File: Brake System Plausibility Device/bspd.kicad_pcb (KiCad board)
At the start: 2 copper layers, 87.9 x 41.3 mm, 29 parts, among them P1 MX150_16, SW1 RESET, U1 MCP604, U2 LM1117-5.0, U3 74LVC2G74, U4 74AUC2G00

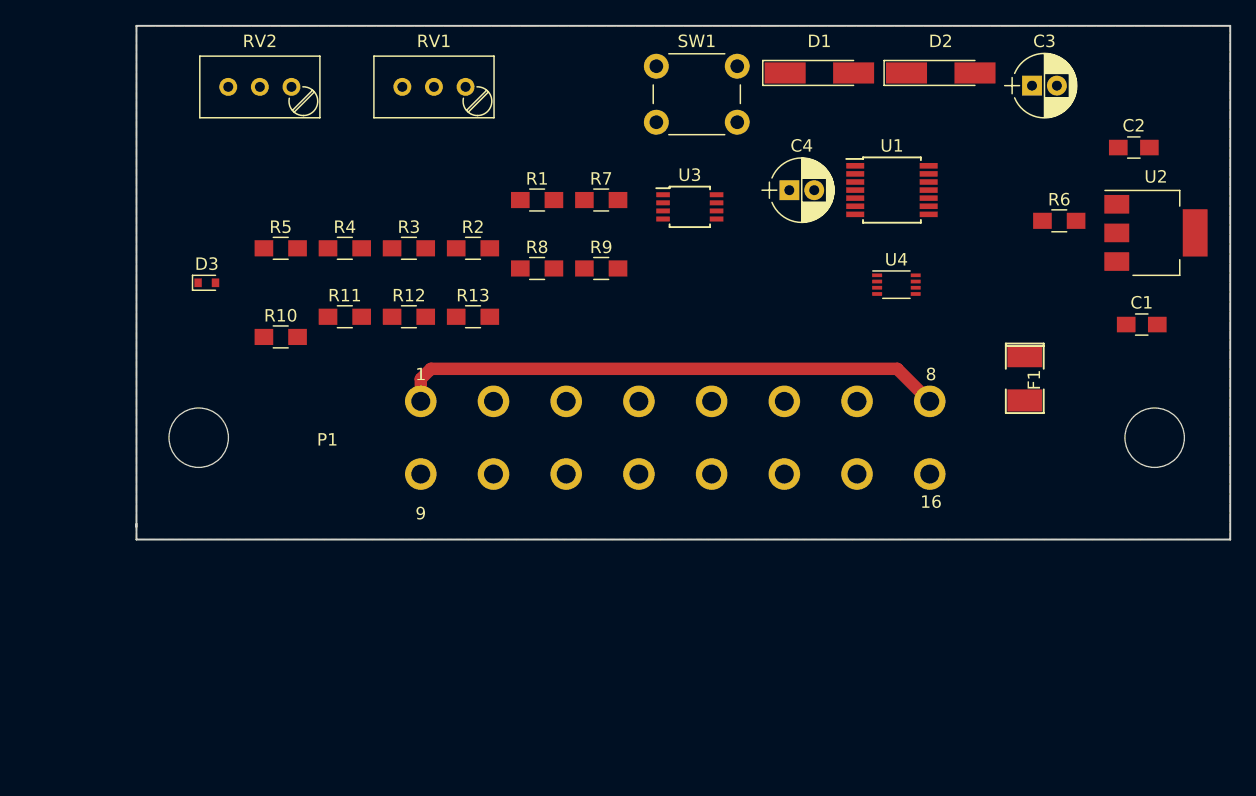
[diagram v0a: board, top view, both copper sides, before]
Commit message: BSPD Layout Done
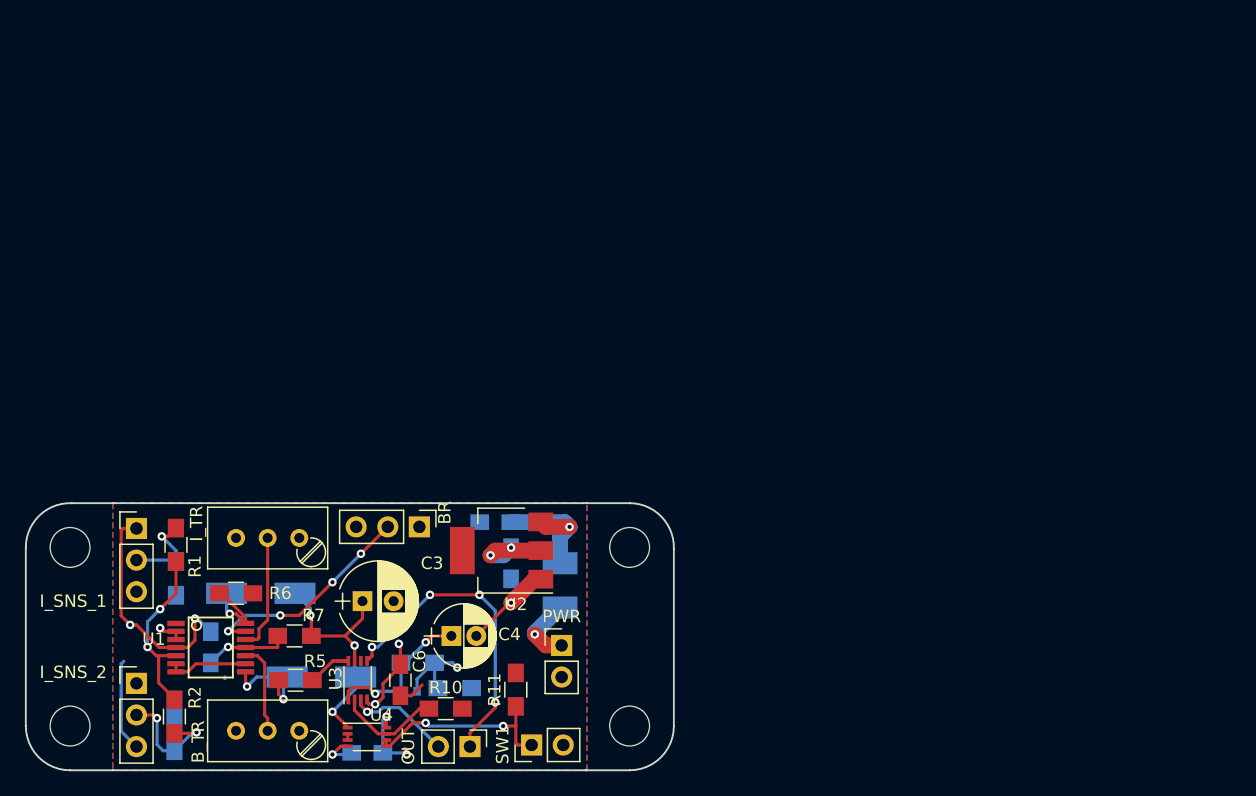
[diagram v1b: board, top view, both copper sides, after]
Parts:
- removed P1: MX150_16, UNCAMotorsports:MX150_16pin
- removed R12, R13: 1k, Resistors_SMD:R_0805_HandSoldering
- removed RV1: 5KW trim - 10k, Potentiometers:Potentiometer_Trimmer_Bourns_3296W
- removed RV2: Braking trim - 10k, Potentiometers:Potentiometer_Trimmer_Bourns_3296W
- added BR: BRAKE_SENSOR, Pin_Headers:Pin_Header_Straight_1x03_Pitch2.54mm, F.Cu at (133.0, 88.8)
- added B_TR: 5KW trim - 10k, Potentiometers:Potentiometer_Trimmer_Bourns_3296W, F.Cu at (123.3, 105.2)
- added C5: 1u, Capacitors_SMD:C_0805_HandSoldering, B.Cu at (116.2, 98.4)
- added C6: 1u, Capacitors_SMD:C_0805_HandSoldering, F.Cu at (131.4, 101.1)
- added C7: 1u, Capacitors_SMD:C_0805_HandSoldering, B.Cu at (128.8, 106.9)
- added I_SNS_1: CURRENT_SENSE_2, Pin_Headers:Pin_Header_Straight_1x03_Pitch2.54mm, F.Cu at (110.2, 88.9)
- added I_SNS_2: CURRENT_SENSE_1, Pin_Headers:Pin_Header_Straight_1x03_Pitch2.54mm, F.Cu at (110.2, 101.3)
- added I_TR: Braking trim - 10k, Potentiometers:Potentiometer_Trimmer_Bourns_3296W, F.Cu at (123.3, 89.7)
- added OUT: Q_QNOT_LATCHED, Pin_Headers:Pin_Header_Straight_1x02_Pitch2.54mm, F.Cu at (137.0, 106.4)
- added PWR: 12V_AND_GND, Pin_Headers:Pin_Header_Straight_1x02_Pitch2.54mm, F.Cu at (144.4, 98.3)
- added REF**: MountingHole_3.2mm_M3, Mounting_Holes:MountingHole_3.2mm_M3, F.Cu at (104.9, 104.8)
- added REF**: MountingHole_3.2mm_M3, Mounting_Holes:MountingHole_3.2mm_M3, F.Cu at (104.9, 90.4)
- added REF**: MountingHole_3.2mm_M3, Mounting_Holes:MountingHole_3.2mm_M3, F.Cu at (149.9, 104.8)
- added REF**: MountingHole_3.2mm_M3, Mounting_Holes:MountingHole_3.2mm_M3, F.Cu at (149.9, 90.4)
- C1, C2, D1, D2, D3, F1, R3, R4, R8, R9: moved to B.Cu
- C3: footprint Capacitors_ThroughHole:CP_Radial_D5.0mm_P2.00mm -> Capacitors_ThroughHole:CP_Radial_D6.3mm_P2.50mm
- R11: value 1k -> 10k
- SW1: value RESET -> SW_Push; footprint Buttons_Switches_ThroughHole:SW_PUSH_6mm -> Pin_Headers:Pin_Header_Straight_1x02_Pitch2.54mm
- U1: footprint Housings_SSOP:TSSOP-14_4.4x5mm_Pitch0.65mm -> SMD_Packages:SSOP-14
- U3: footprint Housings_SSOP:TSSOP-8_3x3mm_Pitch0.65mm -> Housings_SSOP:VSSOP-8_2.3x2mm_Pitch0.5mm
- moved R6 72.6 mm to (118.2, 94.1), turned to 180 degrees
- moved D2 69.5 mm to (125.1, 100.8), turned to 180 degrees
- moved C3 67.9 mm to (128.4, 94.7)
- moved U1 65.9 mm to (116.2, 98.5), turned to 270 degrees
- moved D1 61.3 mm to (120.2, 94.1), turned to 180 degrees
- moved C2 60.2 mm to (140.3, 91.7), turned to 270 degrees
- moved U2 58.4 mm to (139.6, 90.7), turned to 180 degrees
- moved U4 56.0 mm to (128.8, 105.7)
- moved SW1 55.5 mm to (142.0, 106.3), turned to 90 degrees
- moved C1 54.3 mm to (139.1, 88.4), turned to 180 degrees
- moved U3 46.5 mm to (128.0, 101.1), turned to 90 degrees
- moved C4 44.9 mm to (135.5, 97.5)
- moved R2 44.6 mm to (113.3, 104.0), turned to 270 degrees
- moved R7 42.8 mm to (122.9, 97.5), turned to 180 degrees
- moved R4 41.4 mm to (113.3, 105.4), turned to 270 degrees
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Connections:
- R11 pad 1: GND -> Net-(R11-Pad1)
- R11 pad 2: Net-(R11-Pad2) -> +5V
- SW1 pad 1: Net-(R11-Pad2) -> Net-(R11-Pad1)
- SW1 pad 2: +5V -> GND
- U3 pad 3: Net-(R13-Pad2) -> /BSPD_Latched_Output_NOT
- U3 pad 5: /TO_BTS6133 -> /BSPD_Latched_Output
- U4 pad 2: Net-(R11-Pad2) -> Net-(U4-Pad2)
- U4 pad 3: (no net) -> Net-(U4-Pad2)
- U4 pad 5: GND -> Net-(R11-Pad1)
- U4 pad 6: GND -> Net-(R11-Pad1)
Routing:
- net +5V: track 0.00 -> 45.6 mm, vias 0 -> 7
- net +12V: track 44.1 -> 5.53 mm, vias 0 -> 1
- net GND: track 0.00 -> 33.4 mm, vias 0 -> 6
- net /BSPD_Latched_Output: track 0.00 -> 25.5 mm, vias 0 -> 4
- net /BSPD: track 0.00 -> 20.8 mm, vias 0 -> 3
- net /Hard_Braking: track 0.00 -> 17.7 mm, vias 0 -> 4
- net Net-(R11-Pad1): track 0.00 -> 16.1 mm, vias 0 -> 2
- net Net-(R1-Pad2): track 0.00 -> 14.8 mm, vias 0 -> 2
- net Net-(C4-Pad1): track 0.00 -> 12.5 mm, vias 0 -> 2
- net Net-(C1-Pad1): track 0.00 -> 10.6 mm, vias 0 -> 1
- net /Current_R: track 0.00 -> 9.69 mm, vias 0 -> 2
- net Net-(RV2-Pad2): track 0.00 -> 9.45 mm
- net Net-(R10-Pad1): track 0.00 -> 8.46 mm
- net /BSPD_Latched_Output_NOT: track 0.00 -> 8.36 mm, vias 0 -> 1
- net Net-(D2-Pad2): track 0.00 -> 8.35 mm, vias 0 -> 2
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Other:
- board size 87.9 x 41.3 mm -> 52.1 x 21.5 mm
- net class Default: clearance 0.254 -> 0.1524
- rule trace_clearance: 0.254 -> 0.1524
